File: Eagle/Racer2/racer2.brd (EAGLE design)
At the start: 73.3 x 52.1 mm, 8 parts

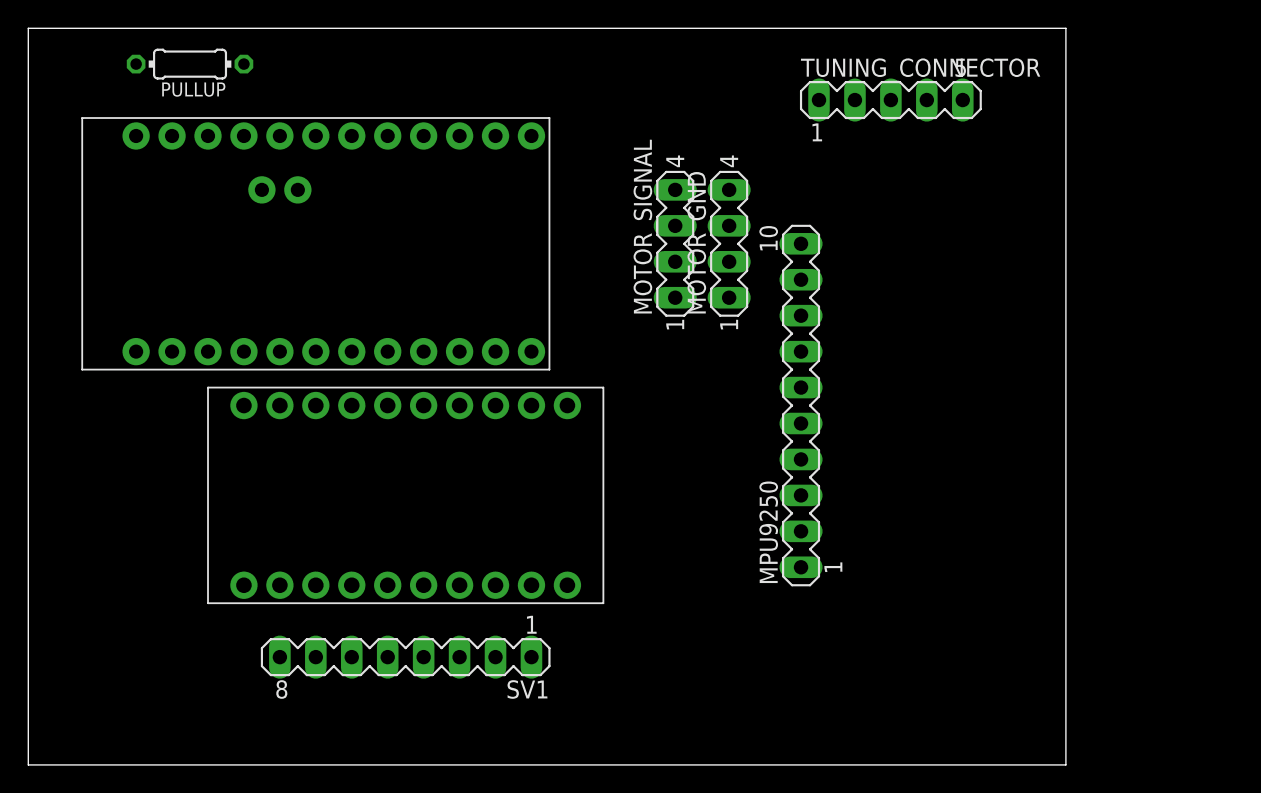
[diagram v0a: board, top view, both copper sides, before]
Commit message: Updated.
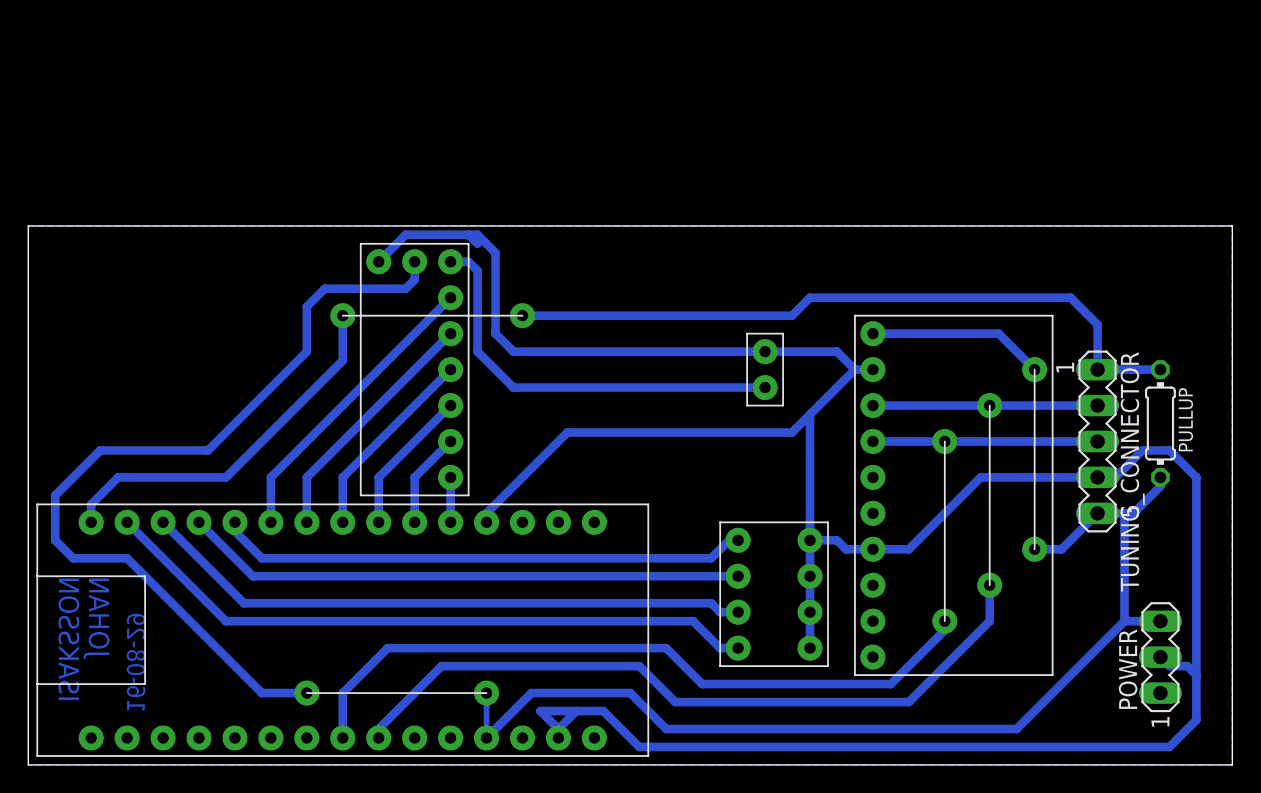
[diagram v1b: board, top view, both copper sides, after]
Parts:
- removed MOTOR_GND, MOTOR_SIGNAL: (no value), con-lstb:MA04-1
- removed MPU9250: (no value), con-lstb:MA10-1
- removed SV1: (no value), con-lstb:MA08-1
- added POWER: (no value), con-lstb:MA03-1
- added U$10, U$6, U$7, U$8, U$9: BRIDGE, quadcopter_comp:BRIDGE
- added U$3: FS_RADIO, quadcopter_comp:FS_RADIO
- added U$4: MPU9250, quadcopter_comp:MPU9250
- added U$5: MOTOR_HEADER, quadcopter_comp:MOTOR_HEADER
- U$1: value SAMD21G_MINI -> NANO; device quadcopter_comp:SAMD21G-MINI -> quadcopter_comp:NANO
- U$2: value LEVELSHIFT_8CH -> BUTTON_PULLUP; device quadcopter_comp:LEVELSHIFT_8CH -> quadcopter_comp:BUTTON_PULLUP
- moved PULLUP 73.1 mm to (80.0, 24.1), turned to 270 degrees
- moved TUNING_CONNECTOR 28.2 mm to (75.6, 22.9), turned to 270 degrees
- moved U$1 27.4 mm to (22.2, 9.53), turned to 270 degrees
- moved U$2 26.9 mm to (52.1, 27.9), turned to 180 degrees
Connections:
- removed net GND2: SV1.8, TUNING_CONNECTOR.4, U$1.GND2, U$2.GND
- removed net N$20: U$1.5, U$2.A5
- removed net N$21: U$1.6, U$2.A4
- removed net N$22: U$1.7, U$2.A3
- removed net N$23: U$1.8, U$2.A2
- removed net N$24: U$1.9, U$2.A1
- new net GND: POWER.2, TUNING_CONNECTOR.4, U$1.GND, U$1.GND2, U$2.B, U$3.GND, U$4.AD0, U$4.GND, U$5.GND1, U$5.GND2, U$5.GND3, U$5.GND4
- new net N$15: U$3.VCC, U$9.A
- new net N$17: U$1.A4, U$6.A
- new net N$8: U$1.D6, U$3.CH5
- net 5V: now also POWER.3, U$1.5V, U$10.B, U$9.B; no longer MPU9250.10, SV1.7, U$1.VIN, U$2.VCCB
- net N$1: now also U$1.D12, U$8.A; no longer MPU9250.7, TUNING_CONNECTOR.3, U$1.SDA
- net N$10: now also U$1.D8, U$5.FL; no longer MOTOR_SIGNAL.2, U$1.12
- net N$11: now also U$1.D9, U$5.FR; no longer SV1.4, U$2.B4
- net N$12: now also U$1.D10, U$5.BL; no longer MOTOR_SIGNAL.4, U$1.10
- net N$13: now also U$1.D11, U$5.BR; no longer SV1.5, U$2.B5
- net N$14: now also U$2.A, U$3.BAT; no longer SV1.6, U$2.B6
- net N$16: now also U$8.B; no longer U$1.2
- net N$18: now also TUNING_CONNECTOR.2, U$4.SCL, U$7.B; no longer U$1.VCC, U$2.VCCA
- net N$19: now also U$10.A, U$4.VCC; no longer U$1.4, U$2.A6
- net N$2: now also U$1.A5, U$7.A; no longer MPU9250.8, TUNING_CONNECTOR.2, U$1.SCL
- net N$3: now also TUNING_CONNECTOR.3, U$4.SDA, U$6.B; no longer MOTOR_GND.1, MOTOR_GND.2, MOTOR_GND.3, MOTOR_GND.4, MPU9250.4, MPU9250.9, U$1.GND
- net N$4: now also U$1.D3, U$3.CH2; no longer SV1.1, U$2.B1
- net N$5: now also U$1.D2, U$3.CH1; no longer MOTOR_SIGNAL.3, U$1.11
- net N$6: now also U$1.D4, U$3.CH3; no longer SV1.2, U$2.B2
- net N$7: now also U$1.D5, U$3.CH4; no longer SV1.3, U$2.B3
- net N$9: now also U$1.D7, U$3.CH6; no longer MOTOR_SIGNAL.1, U$1.13
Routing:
- net GND: track 0.00 -> 195.2 mm
- net 5V: track 0.00 -> 75.3 mm
- net N$15: track 0.00 -> 60.3 mm
- net N$2: track 0.00 -> 51.6 mm
- net N$17: track 0.00 -> 50.3 mm
- net N$16: track 0.00 -> 49.6 mm
- net N$13: track 0.00 -> 46.9 mm
- net N$12: track 0.00 -> 43.3 mm
- net N$11: track 0.00 -> 39.7 mm
- net N$10: track 0.00 -> 37.5 mm
- net N$14: track 0.00 -> 29.3 mm
- net N$1: track 0.00 -> 26.4 mm
- net N$9: track 0.00 -> 21.1 mm
- net N$8: track 0.00 -> 17.5 mm
- net N$3: track 0.00 -> 15.9 mm
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- added copper zone on layer 16, net GND
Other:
- board size 73.3 x 52.1 mm -> 85.1 x 38.1 mm
- board text added: "16-08-29"
- board text added: "JOHAN ISAKSSON"
